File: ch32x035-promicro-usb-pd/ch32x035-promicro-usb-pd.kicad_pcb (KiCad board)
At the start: 2 copper layers, 30 parts, among them J1 USB_TypeC-2.0_Receptacle, SW1 SW_Push, U1 CH32X035G8U6, U3 TPS562203, U4 AMS1117-3.3(NC)

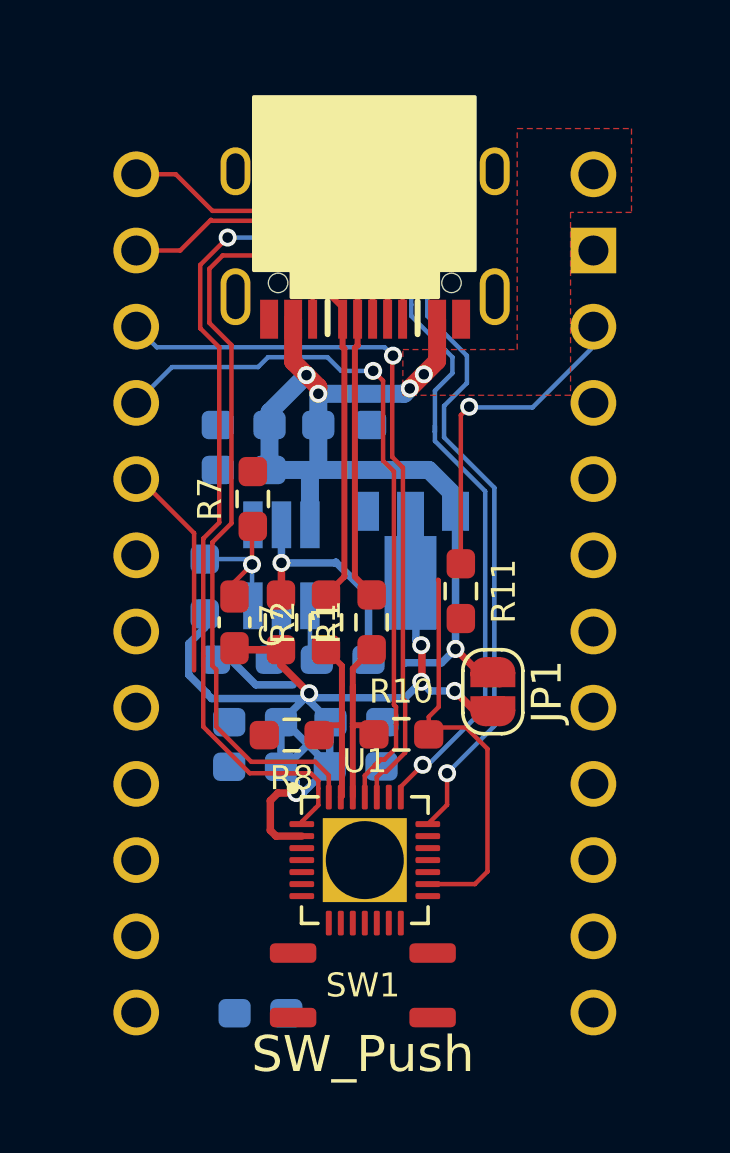
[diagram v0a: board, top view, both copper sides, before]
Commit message: v1.2.0
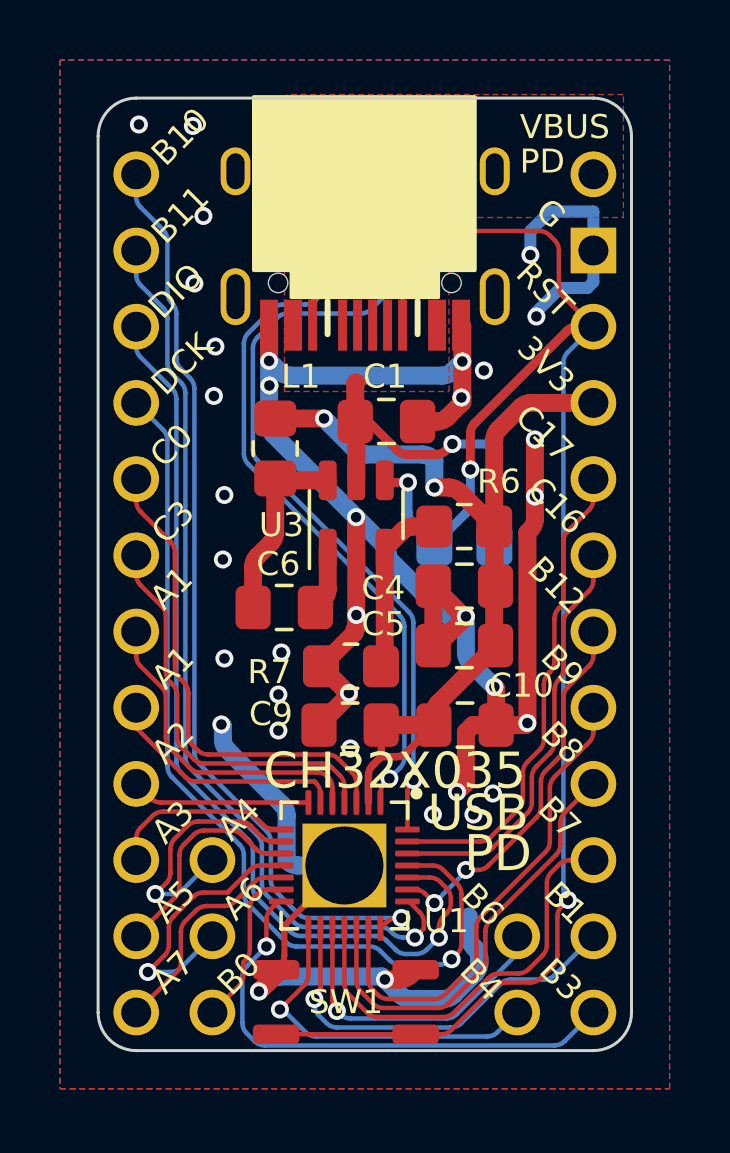
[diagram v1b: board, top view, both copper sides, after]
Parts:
- removed C2: 10u, 74th:Capacitor_0603_1608
- removed C3: 100n, 74th:Capacitor_0603_1608
- removed C7: NC, 74th:Capacitor_0603_1608
- removed JP1: Jumper_2_Open, Jumper:SolderJumper-2_P1.3mm_Open_RoundedPad1.0x1.5mm
- removed R1, R2: 27, 74th:Register_0603_1608
- removed R10, R11, R8: 0(NC), 74th:Register_0603_1608
- removed R3, R4: 5.1k, 74th:Register_0603_1608
- removed R9: 1.5k, 74th:Register_0603_1608
- removed U4: AMS1117-3.3(NC), Package_TO_SOT_SMD:SOT-89-3
- added CH3: 3Pin, 74th:PinOut_3Pin, F.Cu at (76.2, 83.8)
- added CH4: 2Pin, 74th:PinOut_2Pin, F.Cu at (86.4, 86.4)
- added MISC-ACCOUNTTEXT: Logo_74th_text, 74th:Logo_74th_text, B.Cu at (80.3, 73.0)
- added MISC-ICON: LOGO, 74th:Logo_74th_5mm, B.Cu at (79.0, 69.8)
- added REF**: JLCJLCJLCJLC, 74th:Logo_JLCJLCJLCJLC, B.Cu at (75.2, 63.6)
- C1: value 10u -> 22u; footprint 74th:Capacitor_0603_1608 -> 74th:Capacitor_0805_2012; moved to F.Cu
- C10, C4, C5, C6, C9: footprint 74th:Capacitor_0603_1608 -> 74th:Capacitor_0805_2012; moved to F.Cu
- C8: footprint 74th:Capacitor_0603_1608 -> 74th:Capacitor_0805_2012
- CH1: footprint 74th:ProMicro-LIKE_RIGHT -> 74th:PinOut_ProMicro-LIKE_RIGHT
- CH2: footprint 74th:ProMicro-LIKE_LEFT_NO-GND -> 74th:PinOut_ProMicro-LIKE_LEFT_NO-GND
- J1: footprint 74th:USB-C-Receptacle_SMD_12-Pin -> 74th:Connector_USB-C-Receptacle_SMT_12-Pin_Simple
- L1, R5: footprint 74th:Register_0603_1608 -> 74th:Register_0805_2012
- R6: value 135k -> 100k; footprint 74th:Register_0603_1608 -> 74th:Register_0805_2012; moved to F.Cu
- R7: value 30k -> 22k; footprint 74th:Register_0603_1608 -> 74th:Register_0805_2012
- U1: footprint 74th:QFN-28-1EP_4x4mm_P0.4mm_EP2.8x2.8mm_hand-solder -> 74th:Package_QFN-28-1EP_4x4mm_P0.4mm_EP2.8x2.8mm
- U3: value TPS562203 -> MT2492; footprint Package_TO_SOT_SMD:SOT-23-6_Handsoldering -> 74th:Package_SOT-23-6; moved to F.Cu
- moved C8 26.5 mm to (82.6, 62.8)
- moved R6 8.88 mm to (84.6, 72.7), turned to 0 degrees
- moved R5 8.32 mm to (84.6, 73.3), turned to 180 degrees
- moved C4 8.24 mm to (84.6, 74.7)
- moved R7 6.47 mm to (80.8, 77.4), turned to 180 degrees
- moved L1 5.80 mm to (78.3, 70.1), turned to 90 degrees
- moved C5 4.50 mm to (84.6, 76.7), turned to 180 degrees
- moved C10 3.99 mm to (84.6, 79.3)
- moved C9 3.37 mm to (80.8, 79.3)
- moved U3 3.01 mm to (81.0, 72.3), turned to 90 degrees
- moved C6 2.69 mm to (78.6, 75.4), turned to 0 degrees
- moved C1 1.51 mm to (82.0, 69.2)
- moved SW1 0.79 mm to (80.7, 88.5), turned to 180 degrees
- moved U1 0.70 mm to (80.6, 84.0), turned to -90 degrees
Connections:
- C6 pad 2: Net-(U3-BST) -> Net-(U3-BS)
- C8 pad 1: /~{RESET} -> /RESET
- CH1 pad 10: /~{RESET} -> /RESET
- J1 pad 2: Net-(J1-D-) -> unconnected-(J1-D--Pad2)
- J1 pad 3: Net-(J1-D+) -> unconnected-(J1-D+-Pad3)
- R5 pad 2: /~{RESET} -> /RESET
- R6 pad 1: VDD -> /DCDC-FB
- R6 pad 2: Net-(U3-VFB) -> VDD
- R7 pad 1: Net-(U3-VFB) -> /DCDC-FB
- SW1 pad 1: /~{RESET} -> /RESET
- U1 pad 10: /15/SPI_SCK -> /8/A8
- U1 pad 11: /14/SPI_MISO -> /G1
- U1 pad 12: /16/SPI_MOSI -> /9/A9
- U1 pad 13: /2/SDA -> /G2
- U1 pad 14: /4/A6 -> /10/A10
- U1 pad 15: /5 -> /G4
- U1 pad 16: /3/SCL -> /16/SPI_MOSI
- U1 pad 17: /6/A7 -> /G3
- U1 pad 18: Net-(U1-PB7/T1C2N/O2P2/RTS3) -> /14/SPI_MISO
- U1 pad 19: /8/A8 -> /15/SPI_SCK
- U1 pad 20: /9/A9 -> /18/A0
- U1 pad 23: /7 -> /19/A1
- U1 pad 26: /USB_DM -> /20/A2
- U1 pad 27: /USB_DP -> /21/A3
- U1 pad 3: unconnected-(U1-PC0/A10-Pad3) -> /2/SDA
- U1 pad 4: unconnected-(U1-PC3/C1N0/C2N1/C3N1/A13-Pad4) -> /3/SCL
- U1 pad 5: /18/A0 -> /4/A6
- U1 pad 6: /19/A1 -> /5
- U1 pad 7: /20/A2 -> /6/A7
- U1 pad 8: /21/A3 -> /7
- U1 pad 9: /10/A10 -> /G0
- U3 pad 1: GND -> Net-(U3-BS)
- U3 pad 2: Net-(U3-SW) -> GND
- U3 pad 3: VBUS -> /DCDC-FB
- U3 pad 4: Net-(U3-BST) -> /RESET
- U3 pad 5: /~{RESET} -> VBUS
- U3 pad 6: Net-(U3-VFB) -> Net-(U3-SW)
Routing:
- net GND: track 0.00 -> 86.7 mm, vias 0 -> 35
- net /RESET: track 0.00 -> 52.4 mm, vias 0 -> 4
- net VBUS: track 35.1 -> 11.1 mm, vias 5 -> 1
- net /10/A10: track 0.00 -> 17.0 mm, vias 0 -> 1
- net /18/A0: track 0.00 -> 16.1 mm
- net /21/A3: track 0.00 -> 15.9 mm
- net Net-(J1-D+): track 15.9 -> 0.00 mm, vias 2 -> 0
- net Net-(J1-D-): track 14.8 -> 0.00 mm
- net /15/SPI_SCK: track 0.00 -> 14.5 mm
- net /14/SPI_MISO: track 0.00 -> 14.1 mm
- net /20/A2: track 0.00 -> 13.9 mm
- net /~{RESET}: track 13.7 -> 0.00 mm, vias 1 -> 0
- net /16/SPI_MOSI: track 0.00 -> 13.5 mm, vias 0 -> 1
- net /19/A1: track 0.00 -> 12.5 mm, vias 0 -> 2
- net VDD: track 41.8 -> 30.1 mm, vias 5 -> 2
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- added copper zone on B.Cu, net GND
- added copper zone on F.Cu, net GND
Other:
- board outline added: 17.8 x 31.8 mm
- board text added: "3V3"
- board text added: "A1"
- board text added: "A2"
- board text added: "A3"
- board text added: "A4"
- board text added: "A5"
- board text added: "A6"
- board text added: "A7"
- board text added: "B0"
- board text added: "B1"
- board text added: "B10"
- board text added: "B11"
- board text added: "B12"
- board text added: "B3"
- board text added: "B4"
- board text added: "B6"
- board text added: "B7"
- board text added: "B8"
- board text added: "B9"
- board text added: "C0"
- board text added: "C16"
- board text added: "C17"
- board text added: "C3"
- board text added: "CH32X035"
- board text added: "DCK"
- board text added: "DIO"
- board text added: "G"
- board text added: "PD"
- board text added: "RST"
- board text added: "USB"
- board text added: "USB-PD"
- board text added: "VBUS"
- board text added: "v1.0.0"
